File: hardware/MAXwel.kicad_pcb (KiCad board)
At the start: 2 copper layers, 78.7 x 78.1 mm, 137 parts, among them J2 Conn_02x12_Counter_Clockwise, J3 USB_B_Micro, SW1 SW_Push_Dual, SW10 SW_Wuerth_450301014042, SW11 SW_Wuerth_450301014042, SW12 SW_Wuerth_450301014042, SW13 SW_Wuerth_450301014042, SW2 SW_Push_Dual, SW3 SW_Push_Dual, SW4 SW_Push_Dual, SW5 SW_Wuerth_450301014042, SW6 SW_Wuerth_450301014042, SW7 SW_Wuerth_450301014042, SW8 SW_Wuerth_450301014042, U1 D168K, U2 D168K, U3 D168K, U4 D168K, U5 EPM240T100, U6 AMS1117-3.3, X1 50.000, X2 14.756

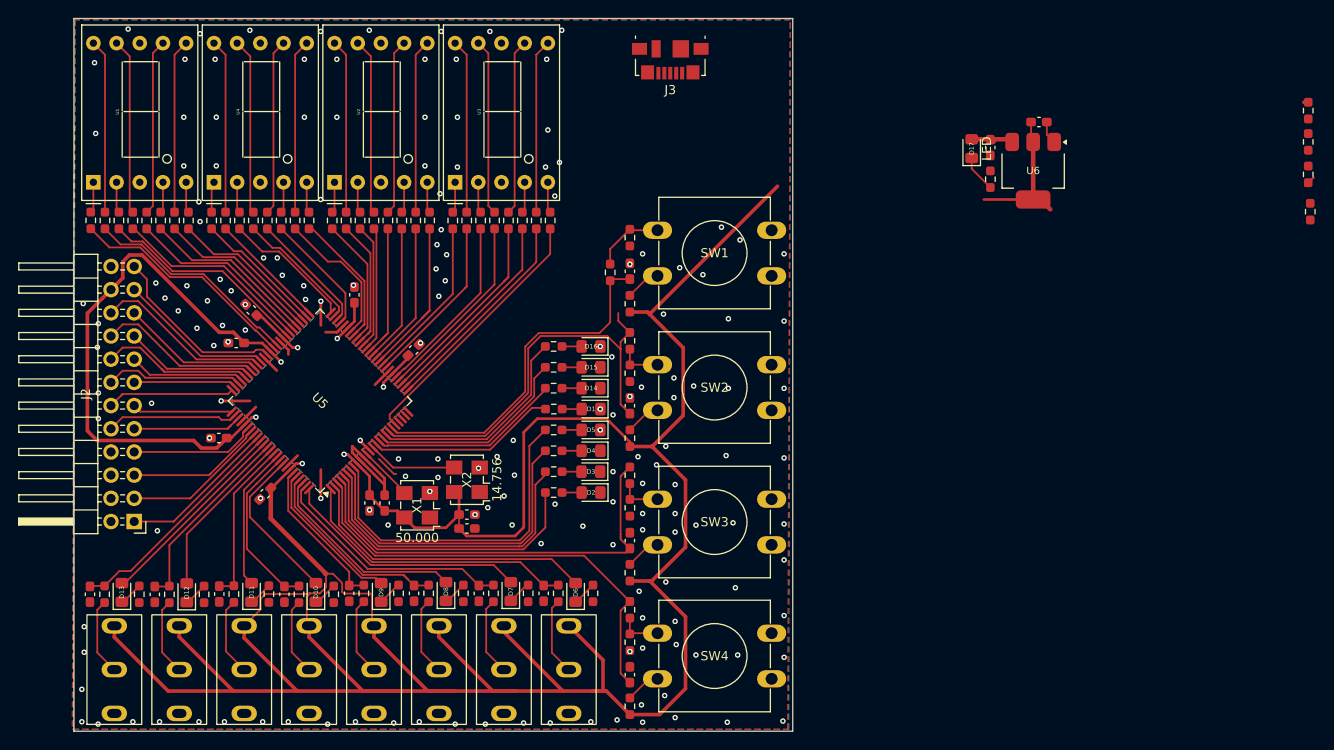
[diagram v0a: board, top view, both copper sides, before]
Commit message: tighter layout
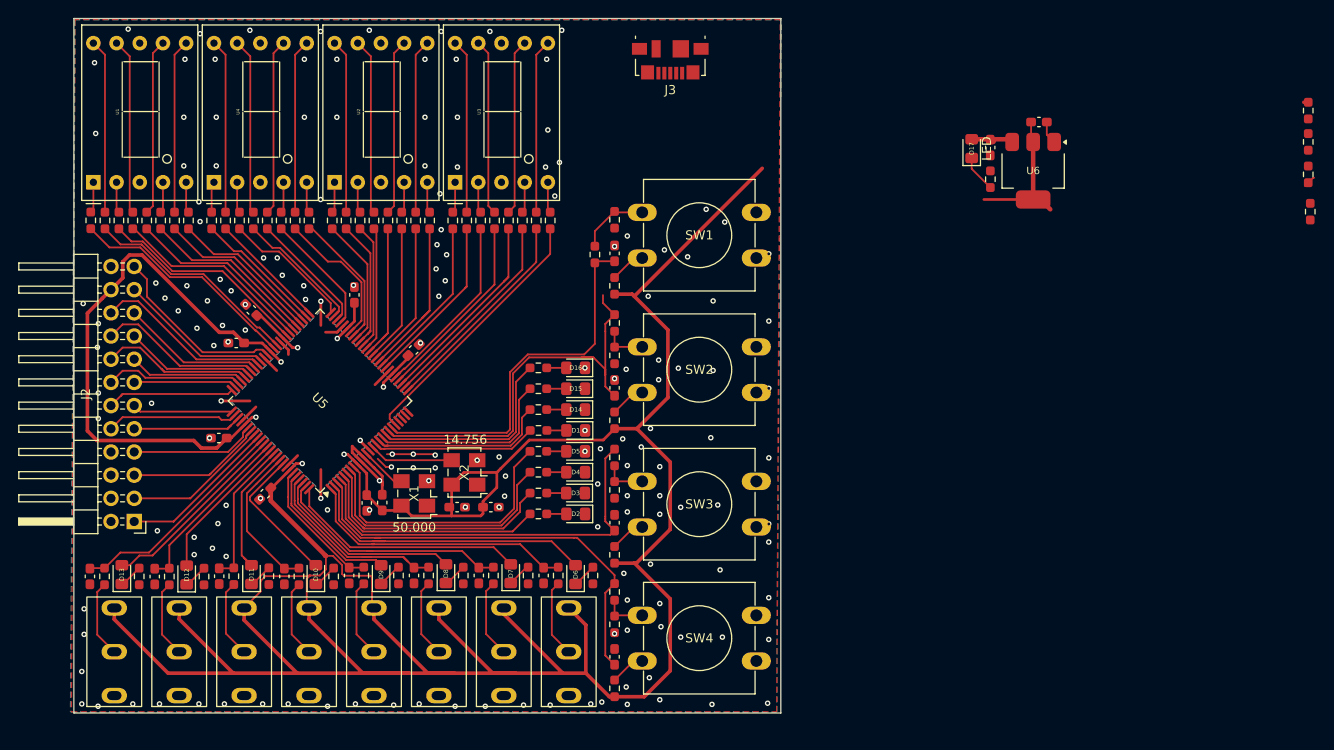
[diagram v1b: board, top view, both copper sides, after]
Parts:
- moved D2 2.88 mm to (160.6, 126.4)
- moved D3 2.88 mm to (160.6, 124.2)
- moved R2 2.88 mm to (156.5, 126.4)
- moved R3 2.88 mm to (156.5, 124.2)
- moved D1 2.88 mm to (160.6, 117.3)
- moved D4 2.88 mm to (160.6, 121.9)
- moved D5 2.88 mm to (160.6, 119.6)
- moved R1 2.88 mm to (156.5, 117.3)
- moved R4 2.88 mm to (156.5, 121.9)
- moved R5 2.88 mm to (156.5, 119.6)
- moved D14 2.88 mm to (160.6, 115.0)
- moved D15 2.88 mm to (160.6, 112.7)
- moved D16 2.88 mm to (160.6, 110.4)
- moved R62 2.88 mm to (156.5, 115.0)
- moved R63 2.88 mm to (156.5, 112.7)
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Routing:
- net +3V3: track 418.3 -> 408.0 mm
- net Net-(U5-IO1_8): track 37.8 -> 30.5 mm
- net Net-(U5-IO1_7): track 36.1 -> 28.9 mm
- net Net-(U5-IO1_6): track 34.5 -> 27.7 mm
- net Net-(U5-IO1_5): track 32.8 -> 26.0 mm
- net GND: track 40.0 -> 43.2 mm, vias 170 -> 172
- net Net-(U5-IO1_4): track 47.6 -> 44.9 mm
- net Net-(U5-IO1_15): track 20.8 -> 18.1 mm
- net Net-(U5-IO1_20): track 38.6 -> 41.0 mm
- net Net-(U5-IO1_17): track 23.0 -> 21.0 mm
- net Net-(U5-IO2_95): track 16.9 -> 15.0 mm
- net Net-(U5-IO2_91): track 18.7 -> 16.7 mm
- net Net-(D12-A): track 18.4 -> 16.4 mm
- net Net-(U5-IO2_87): track 21.3 -> 19.3 mm
- net Net-(U5-IO2_89): track 17.9 -> 16.0 mm
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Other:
- board size 78.7 x 78.1 mm -> 77.4 x 76.1 mm
